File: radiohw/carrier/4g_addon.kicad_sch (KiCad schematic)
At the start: 12 parts, among them J2 Bus_M.2_Socket_B, J7 SIM_Card

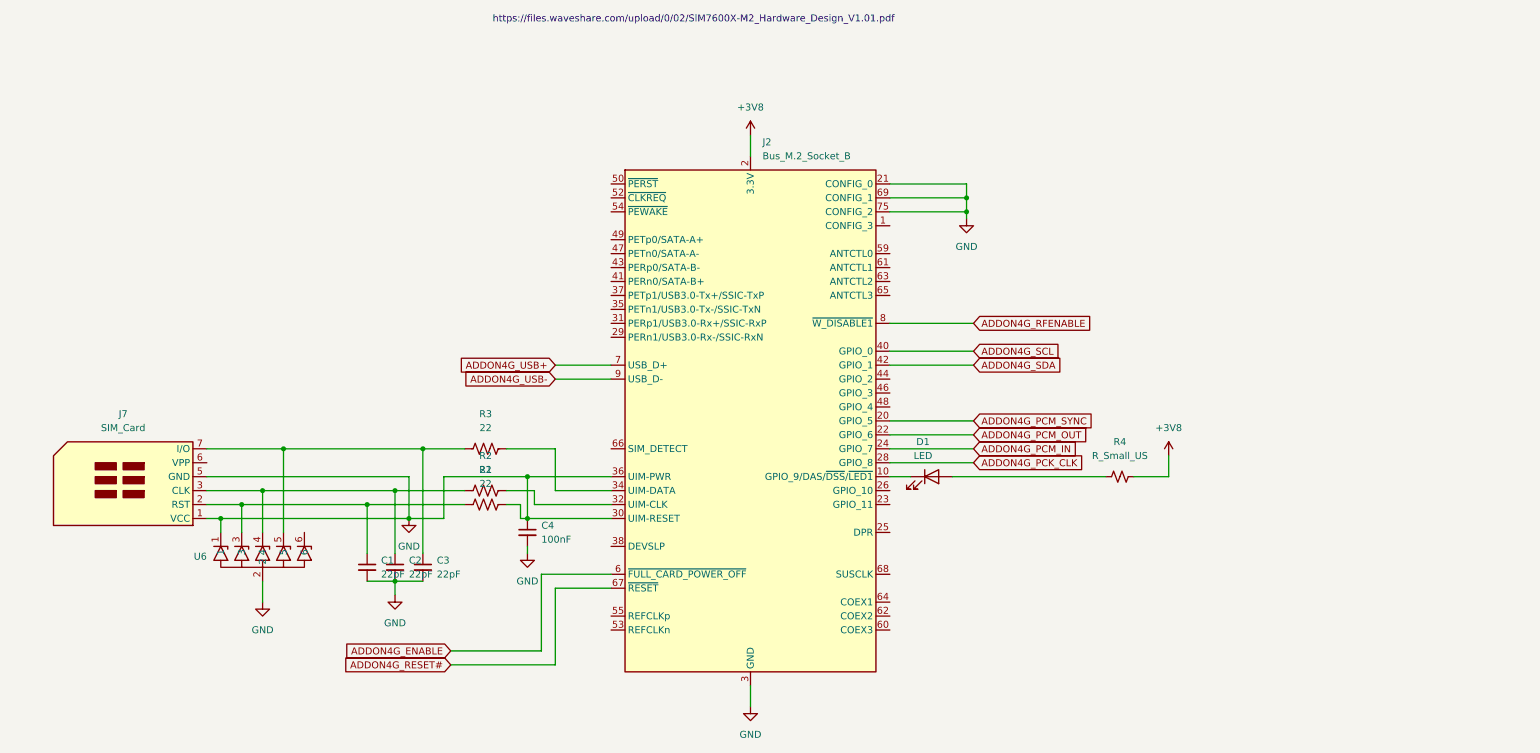
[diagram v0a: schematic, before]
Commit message: Schematic development.
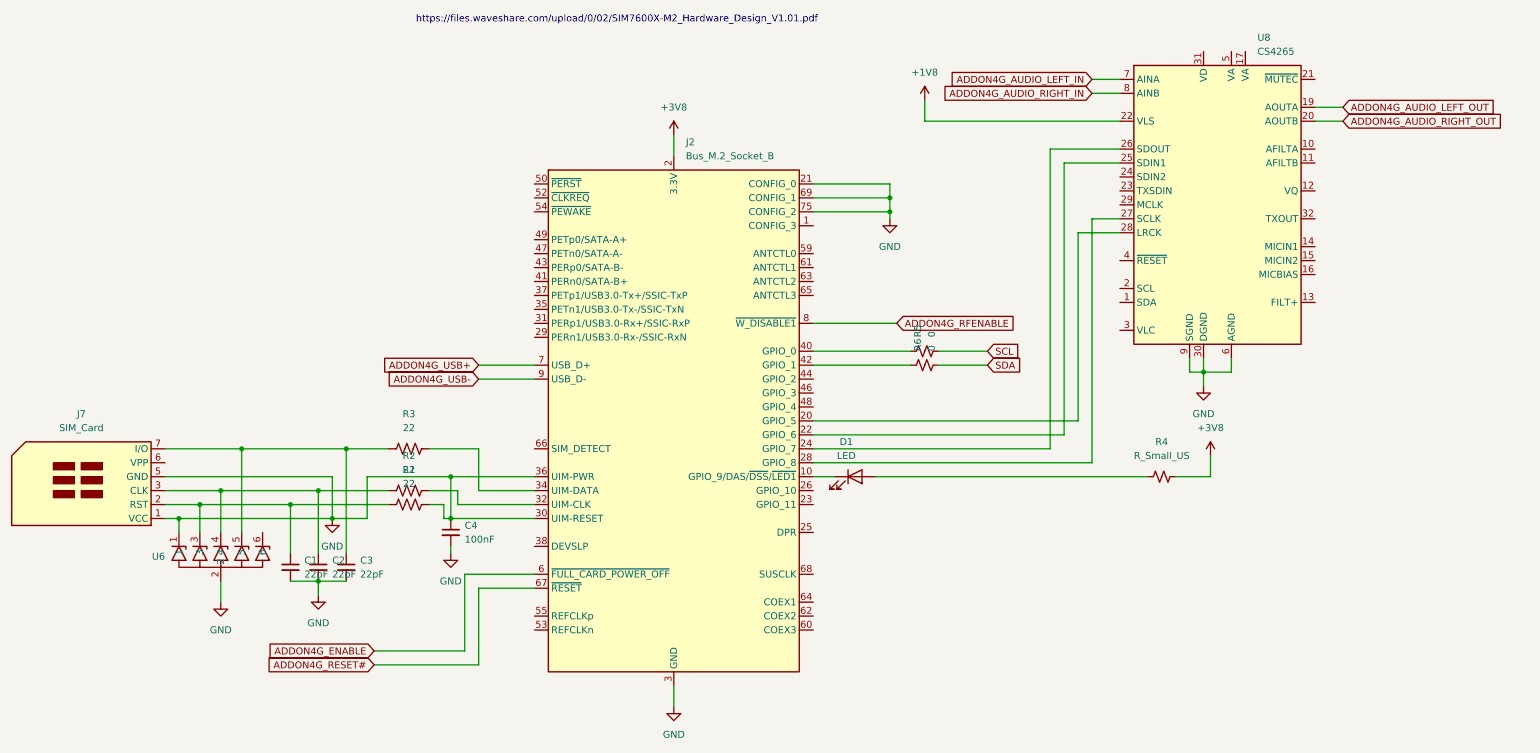
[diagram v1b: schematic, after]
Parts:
- added R5, R6: 0, Resistor_SMD:R_0603_1608Metric_Pad0.98x0.95mm_HandSolder, symbol Device:R_Small_US
- added U8: CS4265, Package_DFN_QFN:QFN-32-1EP_5x5mm_P0.5mm_EP3.6x3.6mm, symbol Audio:CS4265
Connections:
- net GND: now also U8.18 (AGND), U8.30 (DGND), U8.33 (AGND), U8.6 (AGND), U8.9 (SGND)
- net ADDON4G_PCK_CLK: no longer names the net of J2.28 (GPIO_8)
- net ADDON4G_PCK_CLK: now also U8.27 (SCLK)
- net ADDON4G_PCM_IN: no longer names the net of J2.24 (GPIO_7)
- net ADDON4G_PCM_IN: now also U8.26 (SDOUT)
- net ADDON4G_PCM_OUT: no longer names the net of J2.22 (GPIO_6)
- net ADDON4G_PCM_OUT: now also U8.25 (SDIN1)
- net ADDON4G_PCM_SYNC: no longer names the net of J2.20 (GPIO_5)
- net ADDON4G_PCM_SYNC: now also U8.28 (LRCK)
- net ADDON4G_SCL: no longer names the net of J2.40 (GPIO_0)
- net ADDON4G_SCL: now also R5.1
- net ADDON4G_SDA: no longer names the net of J2.42 (GPIO_1)
- net ADDON4G_SDA: now also R6.1
- new net +1V8: U8.22 (VLS)
- new net ADDON4G_AUDIO_LEFT_IN: U8.7 (AINA)
- new net ADDON4G_AUDIO_LEFT_OUT: U8.19 (AOUTA)
- new net ADDON4G_AUDIO_RIGHT_IN: U8.8 (AINB)
- new net ADDON4G_AUDIO_RIGHT_OUT: U8.20 (AOUTB)
- new net SCL: R5.2
- new net SDA: R6.2
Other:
- moved on the sheet: C1, C2, C3, C4, D1, J2, J7, R1, R2, R3, R4, U6
